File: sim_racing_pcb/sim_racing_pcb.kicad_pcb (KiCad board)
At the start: 2 copper layers, 100 x 50 mm, 21 parts, among them J1 Conn_02x04_Socket, U1 A1302KUA-T, U2 A1302KUA-T, U3 LM358, U4 LM1117MP-3.3, U5 LM7805_TO220, U6 Pico

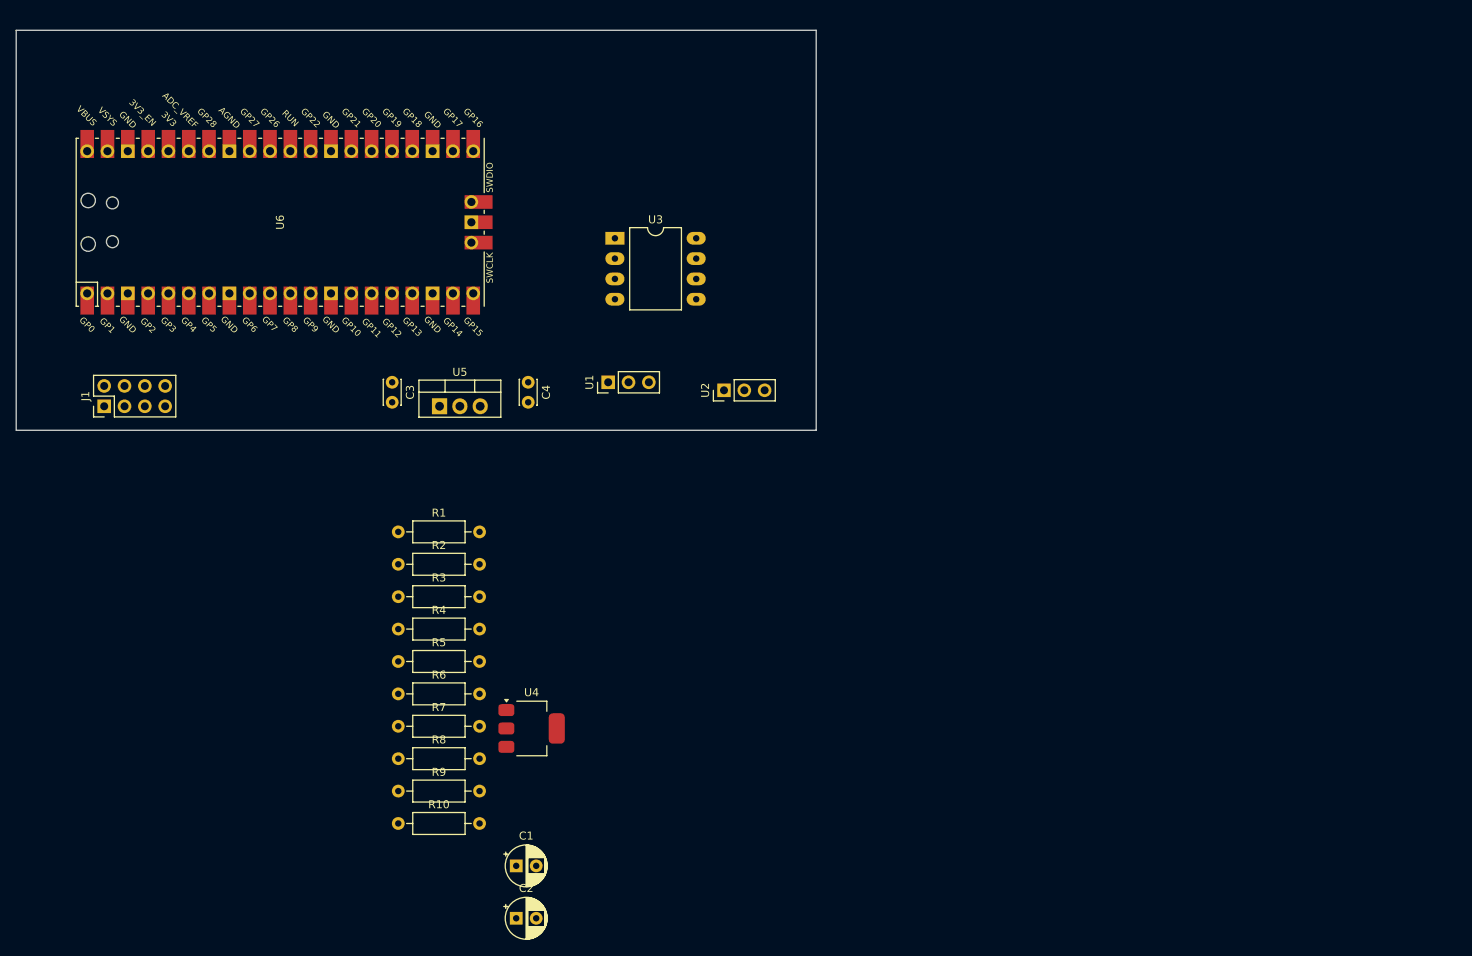
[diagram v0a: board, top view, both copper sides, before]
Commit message: codigo de relleno usb lib en C
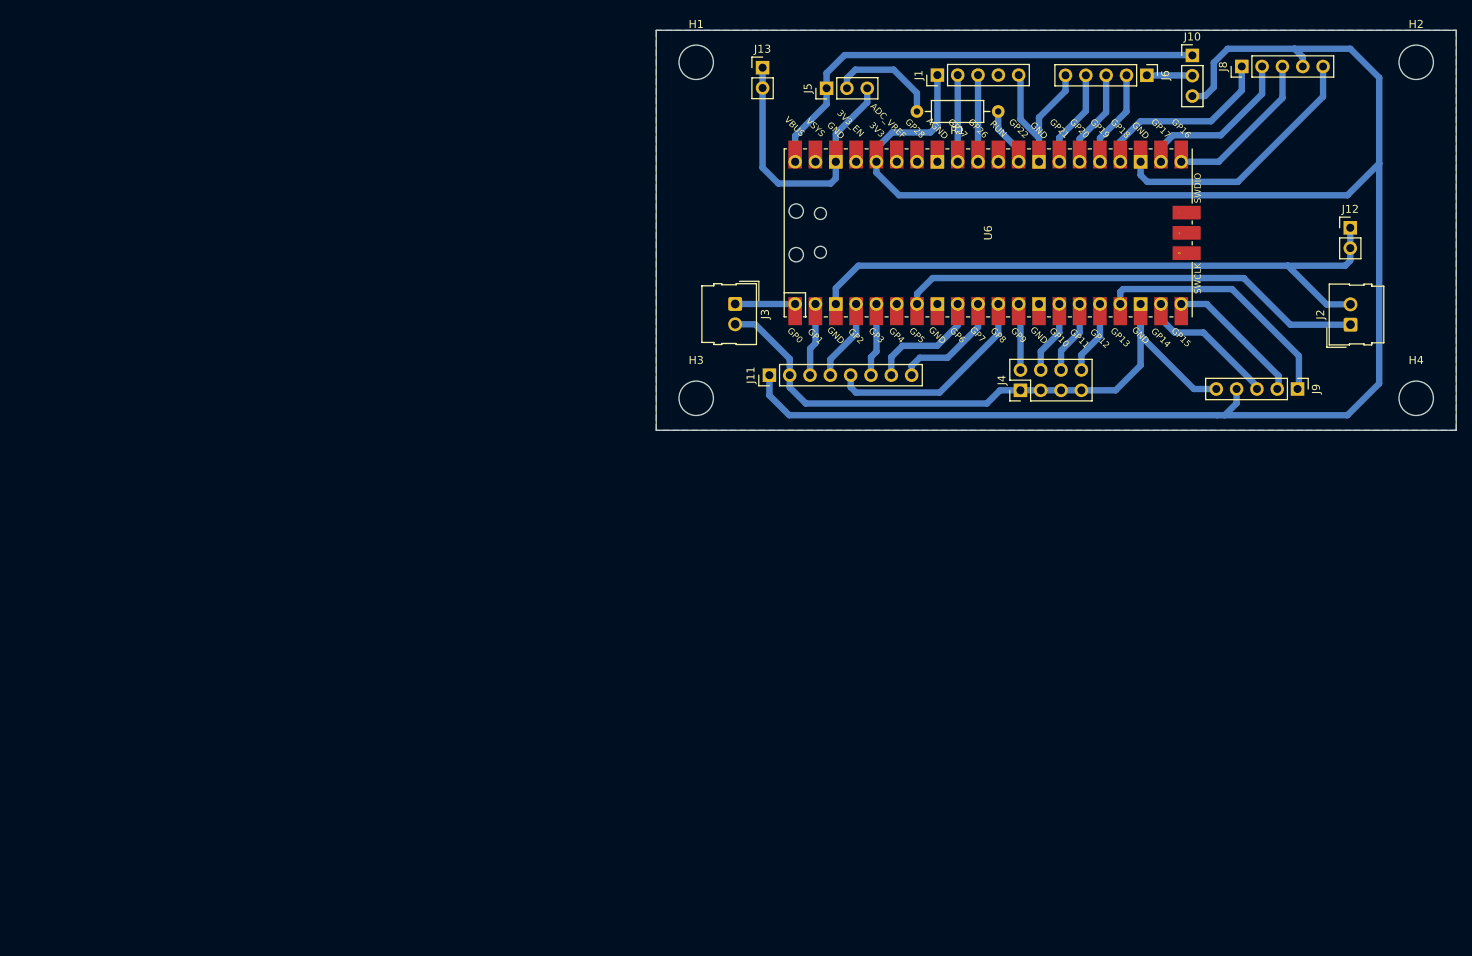
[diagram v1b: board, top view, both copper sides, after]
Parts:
- removed C1, C2: 10uF, Capacitor_THT:CP_Radial_D5.0mm_P2.50mm
- removed C3: 0.33uF, Capacitor_THT:C_Disc_D3.0mm_W2.0mm_P2.50mm
- removed C4: 0.1uF, Capacitor_THT:C_Disc_D3.0mm_W2.0mm_P2.50mm
- removed R10, R4, R5: 10k, Resistor_THT:R_Axial_DIN0207_L6.3mm_D2.5mm_P10.16mm_Horizontal
- removed R2, R8: 2,2k, Resistor_THT:R_Axial_DIN0207_L6.3mm_D2.5mm_P10.16mm_Horizontal
- removed R3, R7, R9: 1k, Resistor_THT:R_Axial_DIN0207_L6.3mm_D2.5mm_P10.16mm_Horizontal
- removed R6: 4,7k, Resistor_THT:R_Axial_DIN0207_L6.3mm_D2.5mm_P10.16mm_Horizontal
- removed U1, U2: A1302KUA-T, Connector_PinHeader_2.54mm:PinHeader_1x03_P2.54mm_Vertical
- removed U3: LM358, Package_DIP:DIP-8_W10.16mm_LongPads
- removed U4: LM1117MP-3.3, Package_TO_SOT_SMD:SOT-223-3_TabPin2
- removed U5: LM7805_TO220, Package_TO_SOT_THT:TO-220-3_Vertical
- added H1: MountingHole, MountingHole:MountingHole_4.3mm_M4_DIN965, F.Cu at (105.0, 24.0)
- added H2: MountingHole, MountingHole:MountingHole_4.3mm_M4_DIN965, F.Cu at (195.0, 24.0)
- added H3: MountingHole, MountingHole:MountingHole_4.3mm_M4_DIN965, F.Cu at (105.0, 66.0)
- added H4: MountingHole, MountingHole:MountingHole_4.3mm_M4_DIN965, F.Cu at (195.0, 66.0)
- added J10: AS5600_POW, Connector_PinHeader_2.54mm:PinHeader_1x03_P2.54mm_Vertical, F.Cu at (167.0, 23.1)
- added J11: Conn_01x08_Pin, Connector_PinHeader_2.54mm:PinHeader_1x08_P2.54mm_Vertical, F.Cu at (114.2, 63.1)
- added J12: Conn_01x02_Pin, Connector_PinHeader_2.54mm:PinHeader_1x02_P2.54mm_Vertical, F.Cu at (186.8, 44.7)
- added J13: Conn_01x02_Pin, Connector_PinHeader_2.54mm:PinHeader_1x02_P2.54mm_Vertical, F.Cu at (113.3, 24.7)
- added J2: Paddle_Shift_R, Connector_Molex:Molex_SL_171971-0002_1x02_P2.54mm_Vertical, F.Cu at (186.8, 56.8)
- added J3: Paddle_Shift_L, Connector_Molex:Molex_SL_171971-0002_1x02_P2.54mm_Vertical, F.Cu at (109.9, 54.2)
- added J4: Conn_02x04_Odd_Even, Connector_PinHeader_2.54mm:PinHeader_2x04_P2.54mm_Vertical, F.Cu at (145.5, 65.0)
- added J5: Leds, Connector_PinHeader_2.54mm:PinHeader_1x03_P2.54mm_Vertical, F.Cu at (121.3, 27.2)
- added J6: AS5600, Connector_PinHeader_2.54mm:PinHeader_1x05_P2.54mm_Vertical, F.Cu at (161.3, 25.6)
- added J8: Encoder - DER, Connector_PinHeader_2.54mm:PinHeader_1x05_P2.54mm_Vertical, F.Cu at (173.2, 24.5)
- added J9: Encoder - MID, Connector_PinHeader_2.54mm:PinHeader_1x05_P2.54mm_Vertical, F.Cu at (180.2, 64.8)
- J1: value Conn_02x04_Socket -> Pedales MicroUsb; footprint Connector_PinHeader_2.54mm:PinHeader_2x04_P2.54mm_Vertical -> Connector_PinHeader_2.54mm:PinHeader_1x05_P2.54mm_Vertical
- R1: value 1k -> 330
- moved J1 112.1 mm to (135.2, 25.6)
- moved R1 91.6 mm to (142.8, 30.1), turned to 180 degrees
- moved U6 88.5 mm to (141.5, 45.3)
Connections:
- J1 pad 1: +5V -> +3V3
- J1 pad 2: +3V3 -> A1-Brk
- J1 pad 3: DIR -> A0-Acc
- J1 pad 4: SDA -> unconnected-(J1-Pin_4-Pad4)
- J1 pad 5: SCL -> GND
- R1 pad 1: Hall_1 -> LEDS
- U6 pad 1: unconnected-(U6-GPIO0-Pad1) -> Shifter_mec_L
- U6 pad 10: unconnected-(U6-GPIO7-Pad10) -> DIS - LED
- U6 pad 11: unconnected-(U6-GPIO8-Pad11) -> DIS - DC
- U6 pad 12: unconnected-(U6-GPIO9-Pad12) -> BTN 1
- U6 pad 13: unconnected-(U6-GND-Pad13) -> GND
- U6 pad 14: unconnected-(U6-GPIO10-Pad14) -> BTN 2
- U6 pad 15: unconnected-(U6-GPIO11-Pad15) -> BTN 3
- U6 pad 16: unconnected-(U6-GPIO12-Pad16) -> BTN 4
- U6 pad 17: unconnected-(U6-GPIO13-Pad17) -> CLK - MID
- U6 pad 18: unconnected-(U6-GND-Pad18) -> GND
- U6 pad 19: unconnected-(U6-GPIO14-Pad19) -> SW - MID
- U6 pad 2: unconnected-(U6-GPIO1-Pad2) -> DIS - CS
- U6 pad 20: unconnected-(U6-GPIO15-Pad20) -> DT - MID
- U6 pad 21: unconnected-(U6-GPIO16-Pad21) -> SW - DER
- U6 pad 22: unconnected-(U6-GPIO17-Pad22) -> DT - DER
- U6 pad 23: unconnected-(U6-GND-Pad23) -> GND
- U6 pad 24: unconnected-(U6-GPIO18-Pad24) -> CLK - DER
- U6 pad 25: unconnected-(U6-GPIO19-Pad25) -> DIR
- U6 pad 26: unconnected-(U6-GPIO20-Pad26) -> SDA
- U6 pad 27: unconnected-(U6-GPIO21-Pad27) -> SCL
- U6 pad 28: unconnected-(U6-GND-Pad28) -> GND
- U6 pad 29: unconnected-(U6-GPIO22-Pad29) -> LEDS
- U6 pad 3: unconnected-(U6-GND-Pad3) -> GND
- U6 pad 31: unconnected-(U6-GPIO26_ADC0-Pad31) -> A0-Acc
- U6 pad 32: unconnected-(U6-GPIO27_ADC1-Pad32) -> A1-Brk
- U6 pad 33: unconnected-(U6-AGND-Pad33) -> GND
- U6 pad 36: unconnected-(U6-3V3-Pad36) -> +3V3
- U6 pad 38: unconnected-(U6-GND-Pad38) -> GND
- U6 pad 4: unconnected-(U6-GPIO2-Pad4) -> DIS - RST
- U6 pad 40: unconnected-(U6-VBUS-Pad40) -> +5V
- U6 pad 5: unconnected-(U6-GPIO3-Pad5) -> DIS - MOSI
- U6 pad 7: unconnected-(U6-GPIO5-Pad7) -> Shifter_mec_R
- U6 pad 8: unconnected-(U6-GND-Pad8) -> GND
- U6 pad 9: unconnected-(U6-GPIO6-Pad9) -> DIS - CLK
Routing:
- net GND: track 0.00 -> 254.1 mm
- net +3V3: track 0.00 -> 239.1 mm
- net +5V: track 0.00 -> 59.4 mm
- net Shifter_mec_R: track 0.00 -> 58.7 mm
- net CLK - MID: track 0.00 -> 31.7 mm
- net DIS - DC: track 0.00 -> 27.0 mm
- net CLK - DER: track 0.00 -> 23.4 mm
- net DT - DER: track 0.00 -> 20.6 mm
- net SW - DER: track 0.00 -> 19.9 mm
- net SW - MID: track 0.00 -> 17.7 mm
- net DT - MID: track 0.00 -> 17.6 mm
- net DIS - CLK: track 0.00 -> 14.9 mm
- net DIS - LED: track 0.00 -> 14.4 mm
- net Net-(J5-Pin_2): track 0.00 -> 14.0 mm
- net SCL: track 0.00 -> 12.2 mm
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- added copper zone on B.Cu, net GND

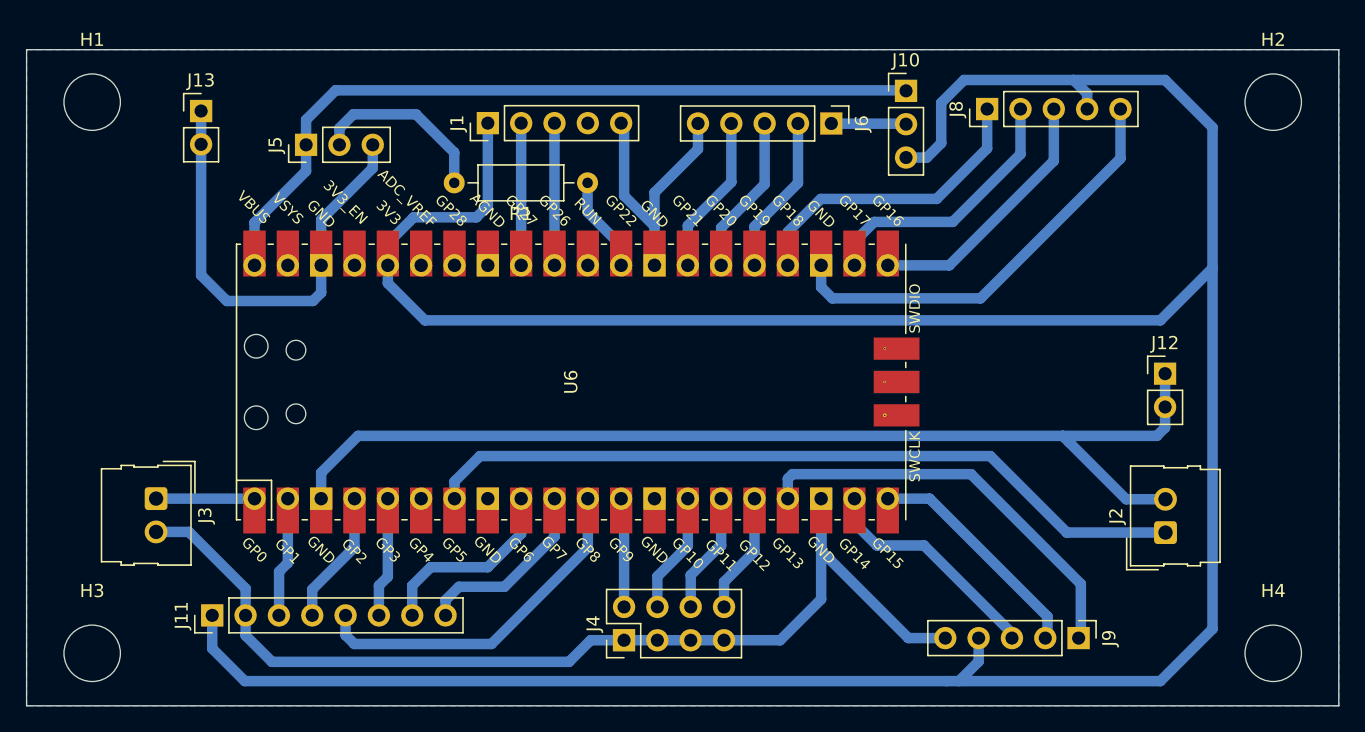
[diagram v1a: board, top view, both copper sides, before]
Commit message: minor changes to pcb
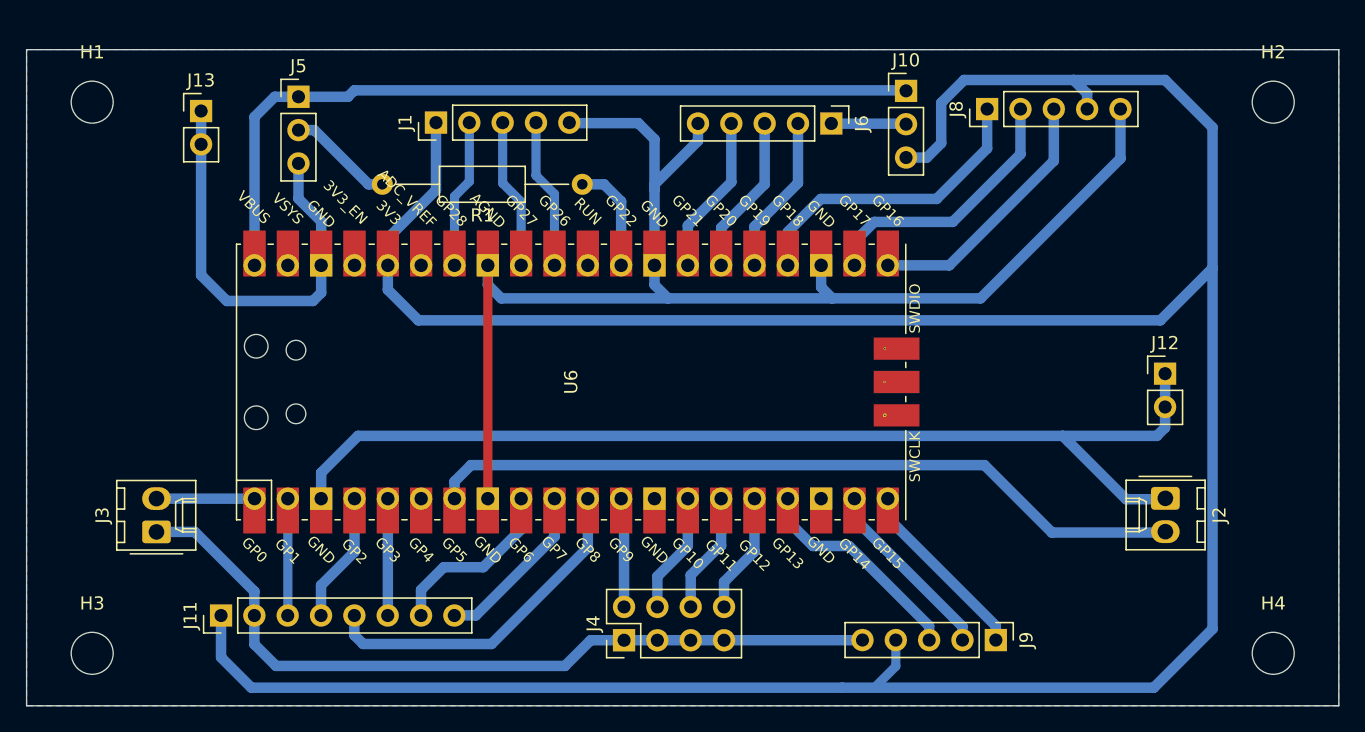
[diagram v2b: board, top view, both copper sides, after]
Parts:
- H1, H2, H3, H4: footprint MountingHole:MountingHole_4.3mm_M4_DIN965 -> MountingHole:MountingHole_3.2mm_M3_DIN965
- J11: value Conn_01x08_Pin -> Display TFT
- J2, J3: footprint Connector_Molex:Molex_SL_171971-0002_1x02_P2.54mm_Vertical -> Connector_Molex:Molex_KK-254_AE-6410-02A_1x02_P2.54mm_Vertical
- R1: footprint Resistor_THT:R_Axial_DIN0207_L6.3mm_D2.5mm_P10.16mm_Horizontal -> Resistor_THT:R_Axial_DIN0207_L6.3mm_D2.5mm_P15.24mm_Horizontal
- moved J9 6.31 mm to (173.9, 65.0)
- moved J1 3.95 mm to (131.2, 25.6)
- moved J5 3.71 mm to (120.7, 23.6), turned to 0 degrees
- moved J2 2.61 mm to (186.8, 54.2), turned to -90 degrees
- moved J3 2.54 mm to (109.9, 56.8), turned to 90 degrees
- moved J11 0.67 mm to (114.8, 63.1)
- moved R1 0.41 mm to (142.3, 30.3)
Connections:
- J1 pad 2: A1-Brk -> A2-Clutch
- J1 pad 3: A0-Acc -> A1-Brk
- J1 pad 4: unconnected-(J1-Pin_4-Pad4) -> A0-Acc
- J2 pad 1: Shifter_mec_R -> GND
- J2 pad 2: GND -> Shifter_mec_R
- J3 pad 1: Shifter_mec_L -> GND
- J3 pad 2: GND -> Shifter_mec_L
- U6 pad 17: CLK - MID -> SW - MID
- U6 pad 19: SW - MID -> DT - MID
- U6 pad 20: DT - MID -> CLK - MID
- U6 pad 34: unconnected-(U6-GPIO28_ADC2-Pad34)_1 -> A2-Clutch
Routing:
- net GND: track 254.1 -> 281.1 mm
- net CLK - MID: track 31.7 -> 14.2 mm
- net A2-Clutch: track 0.00 -> 11.3 mm
- net Net-(J5-Pin_2): track 14.0 -> 8.10 mm
- net DT - MID: track 17.6 -> 14.2 mm
- net +5V: track 59.4 -> 61.8 mm
- net DIS - LED: track 14.4 -> 13.0 mm
- net +3V3: track 239.1 -> 238.0 mm
- net DIS - CLK: track 14.9 -> 13.8 mm
- net LEDS: track 7.35 -> 8.37 mm
- net SW - MID: track 17.7 -> 16.9 mm
- net DIS - DC: track 27.0 -> 26.3 mm
- net A1-Brk: track 10.8 -> 11.5 mm
- net A0-Acc: track 10.8 -> 11.5 mm
- net Shifter_mec_R: track 58.7 -> 58.1 mm
